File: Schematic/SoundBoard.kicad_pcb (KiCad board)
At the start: 2 copper layers, 59 parts, among them J1 Conn_ARM_JTAG_SWD_10, J2 Micro_SD_Card, J3 USB_B_Micro, SW1 SW_Push, SW2 SW_Push, U1 STM32F427VGTx, U2 AH1806-W, U3 FT232RL, U4 TPA301DR, U5 MCP73812T-420I-OT, U6 STC3100IST, U7 MIC5504-3.3YM5, U8 MIC5504-3.3YM5

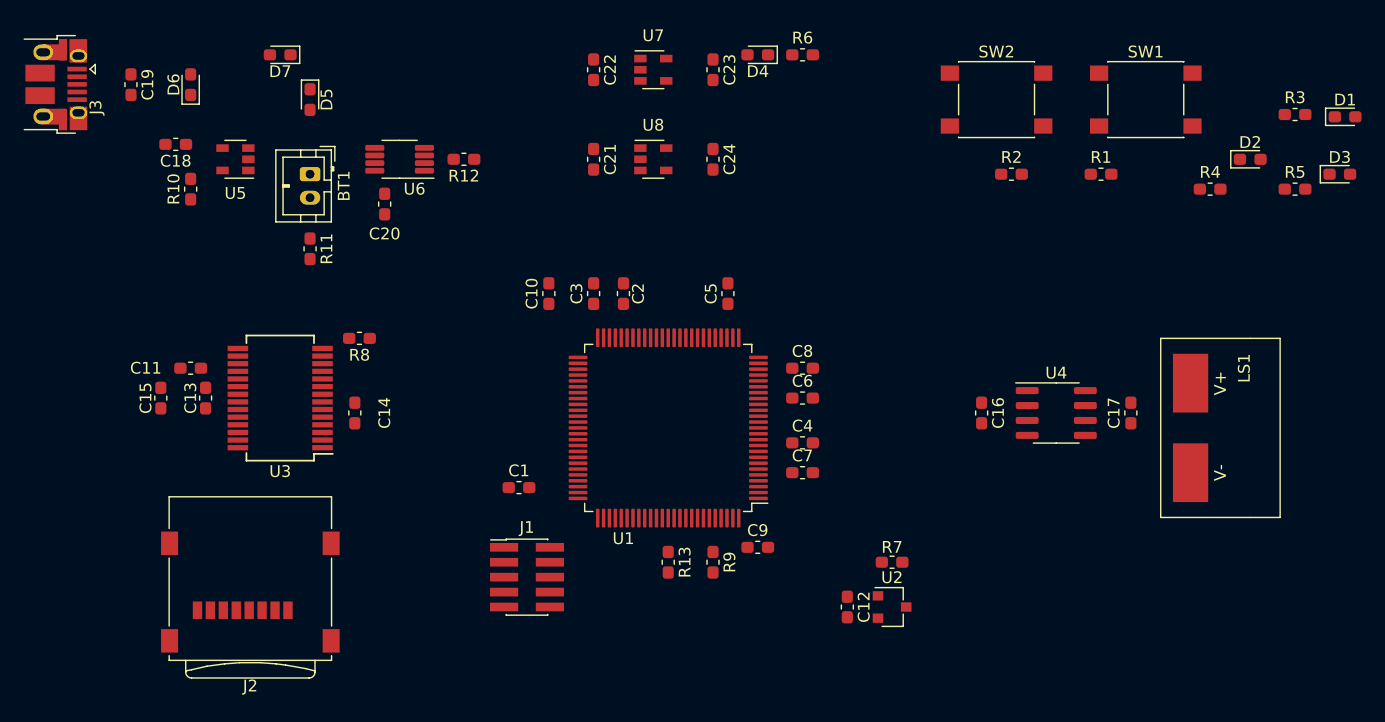
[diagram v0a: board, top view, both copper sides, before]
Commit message: Preliminary routing
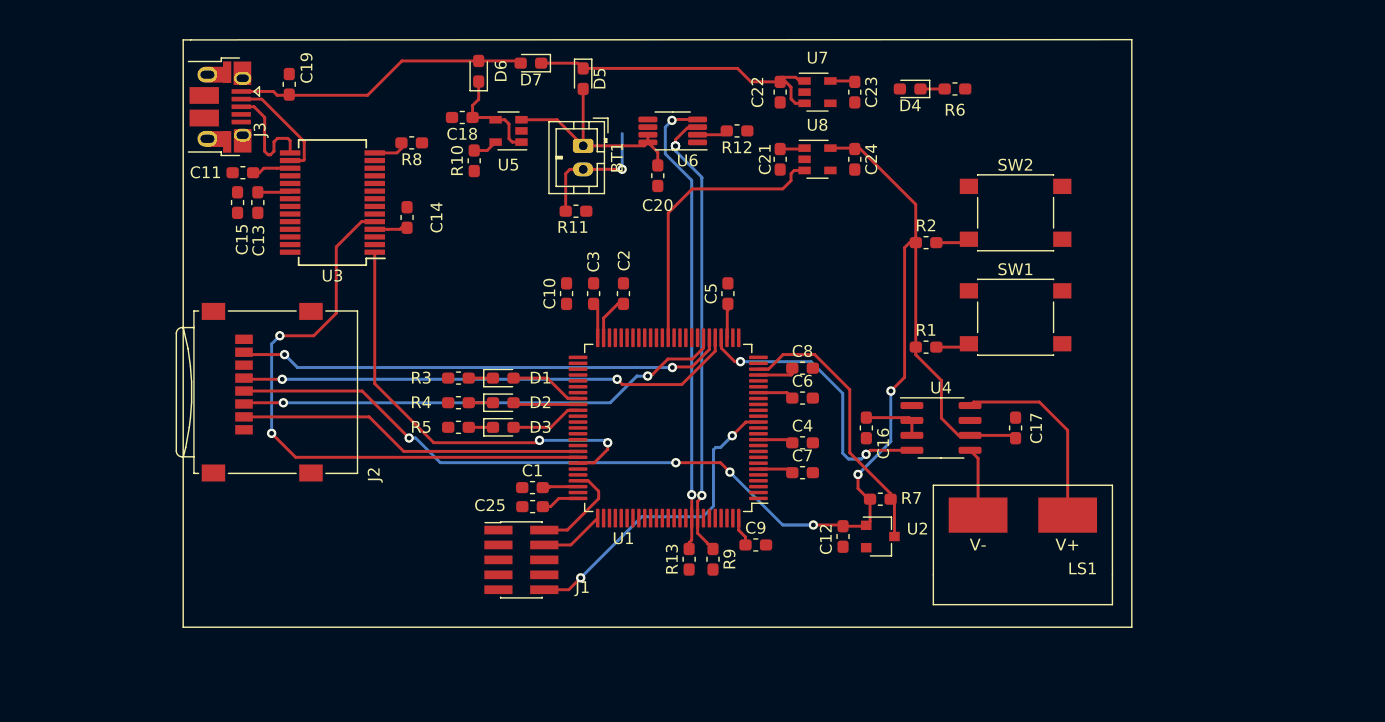
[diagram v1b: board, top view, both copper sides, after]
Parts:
- added C25: 100nF, Capacitor_SMD:C_0603_1608Metric_Pad1.05x0.95mm_HandSolder, F.Cu at (71.0, 72.7)
- moved D1 75.0 mm to (68.5, 61.8)
- moved R3 74.6 mm to (64.7, 61.8), turned to 180 degrees
- moved D3 74.4 mm to (68.5, 66.0)
- moved R5 74.0 mm to (64.7, 66.0), turned to 180 degrees
- moved D2 66.9 mm to (68.5, 63.9)
- moved R4 66.5 mm to (64.7, 63.9), turned to 180 degrees
- moved D6 24.5 mm to (66.4, 35.7)
- moved C18 24.5 mm to (65.0, 39.6)
- moved R10 24.3 mm to (66.0, 43.3)
- moved BT1 23.4 mm to (75.3, 42.0)
- moved C20 23.4 mm to (81.7, 44.6)
- moved R12 23.4 mm to (88.4, 40.8)
- moved U5 23.4 mm to (69.0, 40.8)
- moved U6 23.4 mm to (82.9, 40.8)
- moved D5 23.3 mm to (75.3, 36.3)
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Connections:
- C7 pad 1: /MCU/VDD -> GND
- C7 pad 2: GND -> /MCU/VDD
- R1 pad 1: /MCU/VDD -> /Audio/V1
- R2 pad 1: /MCU/VDD -> /Audio/V1
- U1 pad 38: Net-(U1-Pad38) -> /MCU/V1_EN
- U1 pad 66: /MCU/V1_EN -> Net-(U1-Pad66)
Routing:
- net /Audio/V1: track 0.00 -> 120.1 mm, vias 0 -> 6
- net /MCU/TX_FROM_STM32: track 0.00 -> 50.9 mm, vias 0 -> 2
- net /MCU/SD_CLK: track 0.00 -> 42.6 mm, vias 0 -> 2
- net /MCU/SD_MOSI: track 0.00 -> 41.9 mm, vias 0 -> 2
- net /MCU/SD_MISO: track 0.00 -> 41.8 mm, vias 0 -> 2
- net /MCU/FUEL_SCL: track 0.00 -> 39.9 mm, vias 0 -> 2
- net /MCU/FUEL_SDA: track 0.00 -> 39.6 mm, vias 0 -> 3
- net /MCU/RX_TO_STM32: track 0.00 -> 36.8 mm, vias 0 -> 2
- net /MCU/VDD: track 0.00 -> 32.1 mm
- net /MCU/SD_SELECT: track 0.00 -> 29.6 mm
- net /Power/VRAW: track 0.00 -> 29.1 mm
- net /MCU/NRESET: track 0.00 -> 26.9 mm, vias 0 -> 2
- net Net-(C19-Pad1): track 0.00 -> 25.2 mm
- net /Audio/AUDIO_FROM_DAC: track 0.00 -> 24.3 mm, vias 0 -> 2
- net /MCU/V1_EN: track 0.00 -> 24.1 mm
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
